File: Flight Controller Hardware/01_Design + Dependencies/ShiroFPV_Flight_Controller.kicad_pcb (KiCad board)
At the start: 4 copper layers, 40 x 40 mm, 116 parts, among them J1 GND, J10 TLM, J11 Video_Out, J12 Video_IN, J13 5V3, J14 RX3, J15 TX3, J16 GND3, J17 5V4, J18 RX4, J19 TX4, J2 GND, J20 GND4, J24 +5V, J25 RSSI, J26 GND5, J29 SBUS, J3 VBAT, J30 5V5, J31 RX5, J32 TX5, J33 RX6, J34 5V6, J35 GND6, J36 TX6, J37 10V, J38 RX1, J39 TX1, J4 VBAT, J40 GND1, J42 B-, J46 GND, J5 M1, J6 M2, J7 M3, J8 M4, J9 CUR, P1 USB_C_Plug_USB2.0, Q1 AO3401A, Q2 AO3400A, Q3 BC817W, U1 AT32F435RGT7, U10 AT7456, U3 ICM-20602, U4 BME280, U5 TPS54302, U6 TPS54302DDCR, U7 RT9013-33GB, U8 W25Q128JVS, Y2 27MHz

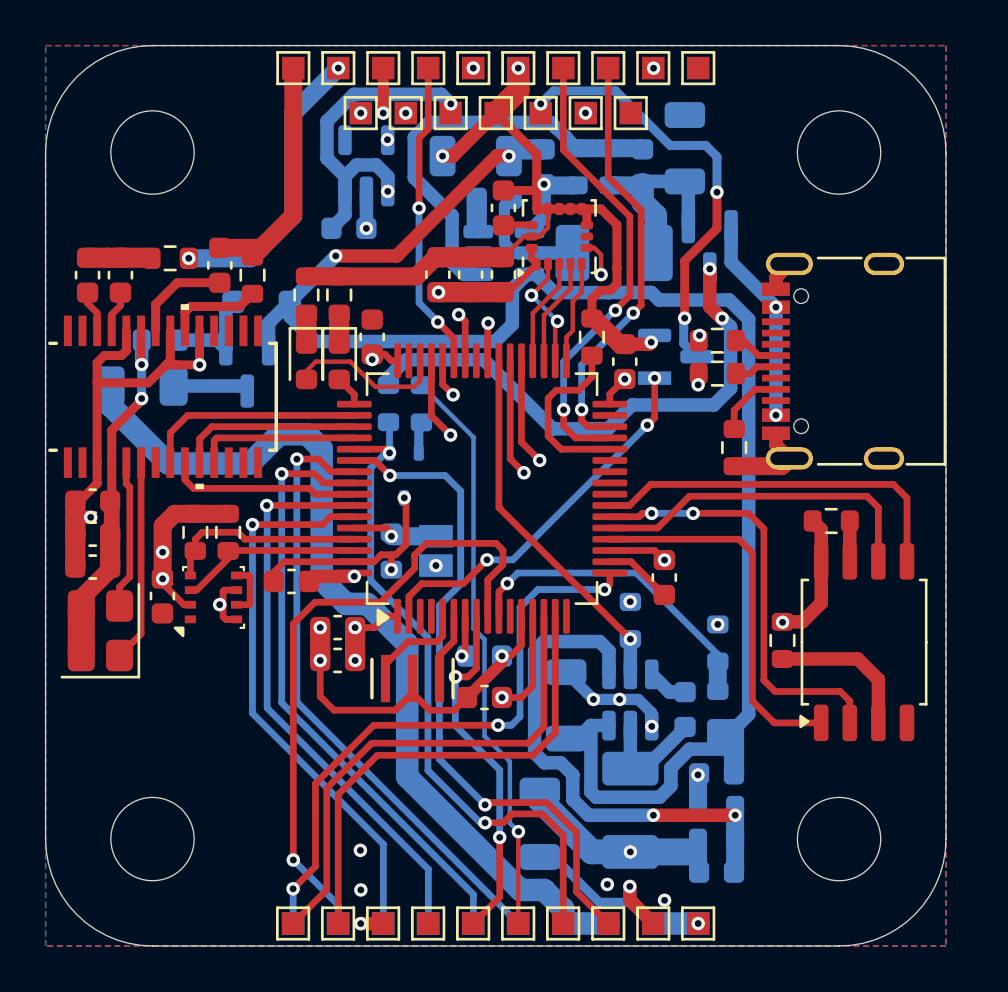
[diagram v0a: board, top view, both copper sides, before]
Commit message: Lots of new stuff
Added a new Website thus it not beeing finished yet.
and updated the PCB
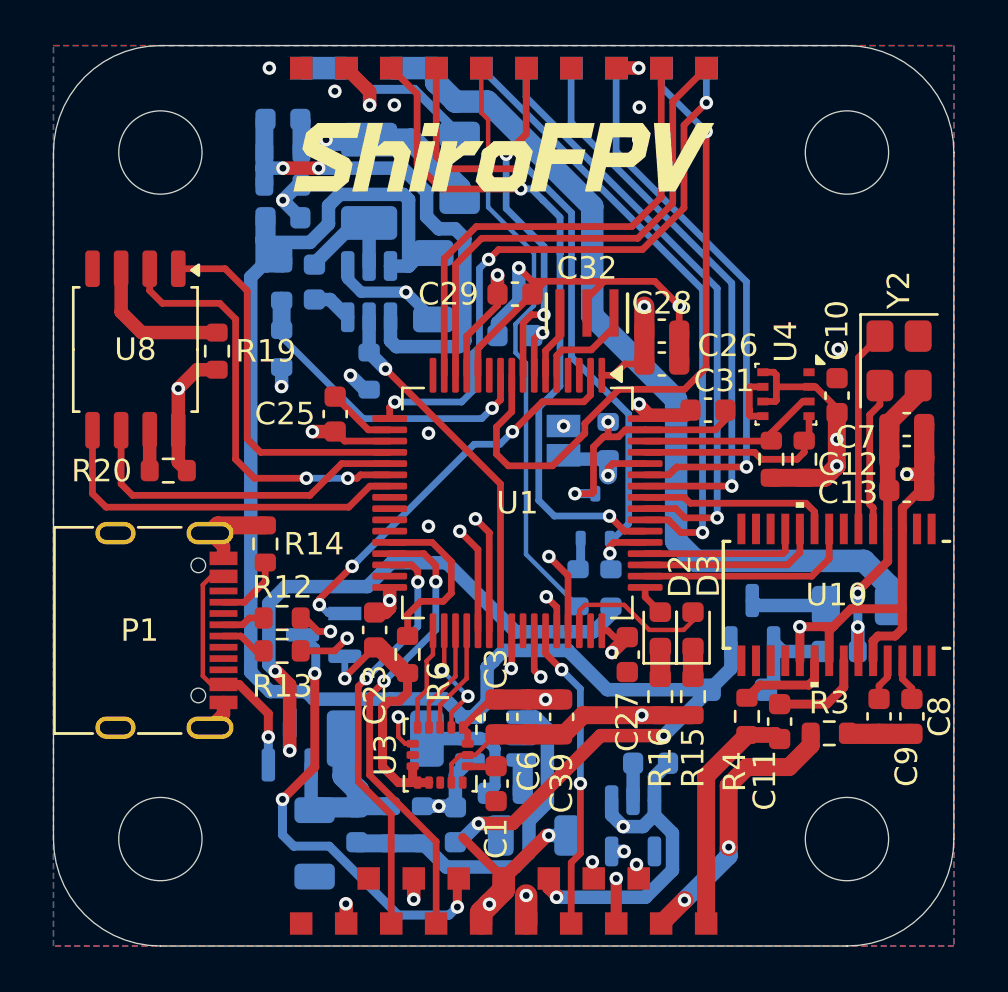
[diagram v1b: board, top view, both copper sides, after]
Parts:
- added G***: LOGO, LOGO, F.Cu at (202.2, 75.5)
- J1, J10, J11, J12, J13, J14, J15, J16, J17, J18, J19, J2, J20, J24, J25, J26, J29, J3, J30, J31, J32, J33, J34, J35, J36, J37, J38, J39, J4, J40, J42, J46, J5, J6, J7, J8, J9: footprint TestPoint:TestPoint_Pad_1.0x1.0mm -> TestPoint:TestPoint_Pad_1.0x1.0mm_No_Silkscreen
- moved REF** 43.4 mm to (217.4, 75.3), turned to 90 degrees
- moved REF** 43.4 mm to (217.4, 105.8), turned to 90 degrees
- moved REF** 42.9 mm to (186.9, 105.8), turned to 90 degrees
- moved REF** 42.9 mm to (186.9, 75.3), turned to 90 degrees
- moved J10 42.2 mm to (211.2, 71.5), turned to -90 degrees
- moved J19 42.2 mm to (211.2, 71.5), turned to 90 degrees
- moved J12 42.2 mm to (211.2, 109.5), turned to 90 degrees
- moved J46 41.9 mm to (193.2, 109.5), turned to 90 degrees
- moved J1 41.9 mm to (193.2, 71.5), turned to -90 degrees
- moved J40 41.9 mm to (193.2, 71.5), turned to 90 degrees
- moved C8 41.5 mm to (220.3, 100.3), turned to -90 degrees
- moved J18 40.6 mm to (209.2, 71.5), turned to 90 degrees
- moved J9 40.6 mm to (209.2, 71.5), turned to -90 degrees
- moved J11 40.6 mm to (209.2, 109.5), turned to 90 degrees
- moved J17 40.4 mm to (195.2, 71.5), turned to 90 degrees
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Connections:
- Y2 pad 3: (no net) -> GND
- Y2 pad 4: (no net) -> GND
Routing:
- net +3.3V: track 37.5 -> 45.5 mm, vias 15 -> 13
- net +5V: track 62.4 -> 66.8 mm
- net GND: track 120.2 -> 123.3 mm, vias 22 -> 20
- net Net-(U5-FB): track 18.6 -> 15.6 mm
- net VBUS: track 9.20 -> 11.0 mm, vias 2 -> 1
- net USBD+: track 17.9 -> 16.5 mm
- net VBAT: track 40.8 -> 39.4 mm
- net BEEPER: track 16.9 -> 18.2 mm
- net BEEPER_B-: track 19.4 -> 20.4 mm
- net BOOT0: track 3.88 -> 4.83 mm
- net ADC_CURRENT: track 28.6 -> 29.5 mm
- net +10V: track 47.3 -> 48.1 mm, vias 2 -> 4
- net V_IN: track 11.6 -> 10.7 mm
- net SBUS: track 25.7 -> 26.4 mm
- net UART5RX: track 29.6 -> 30.2 mm
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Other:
- outline, holes or cut-outs redrawn
- board text added: "Front"
- board text added: "R13"
